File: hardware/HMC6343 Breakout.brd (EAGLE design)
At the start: 20.3 x 20.3 mm, 15 parts, among them U1 HMC6343A

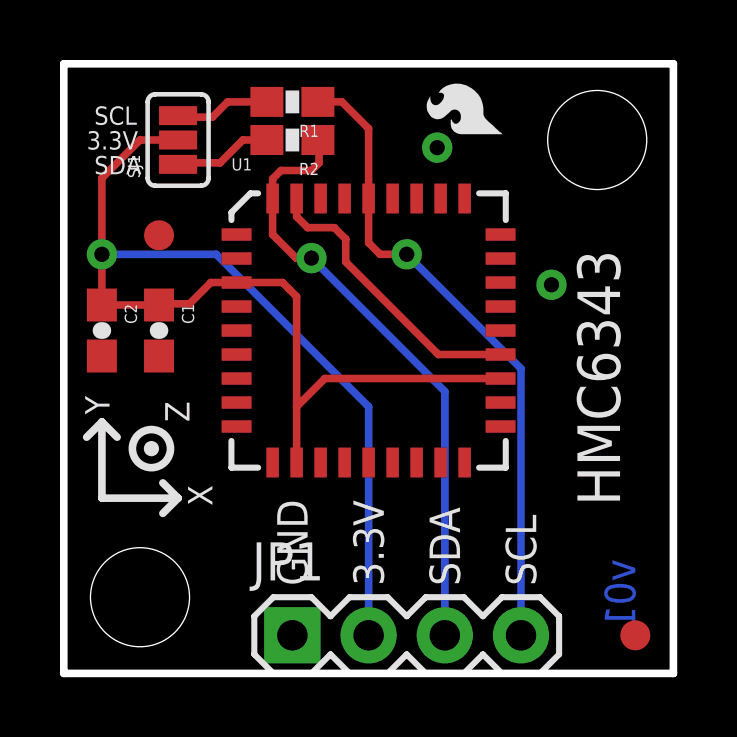
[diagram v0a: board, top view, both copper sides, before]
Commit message: v10, ready for reds
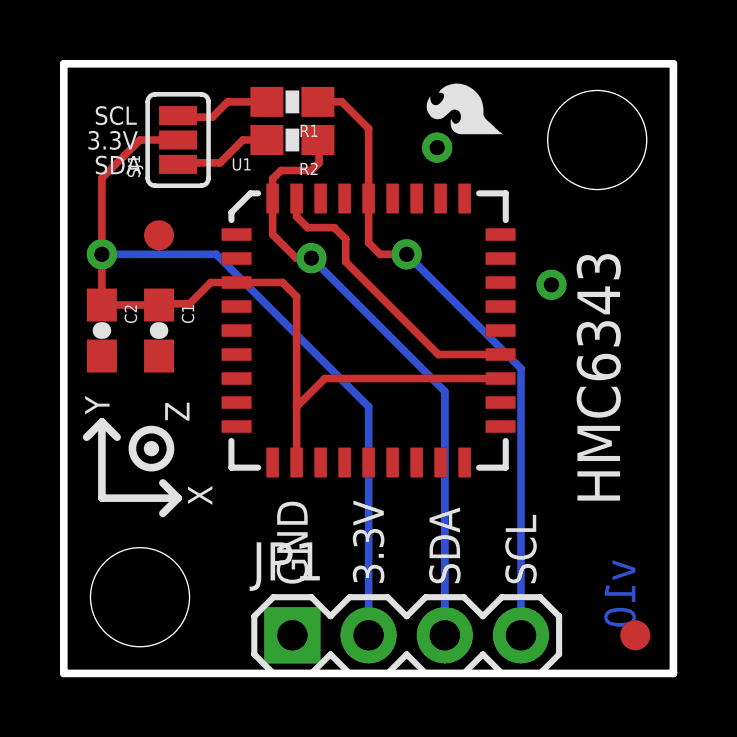
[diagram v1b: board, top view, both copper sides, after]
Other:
- board text added: "v10"
- board text removed: "v01"
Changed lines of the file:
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@@
 <text x="13.335" y="15.24" size="1.016" layer="22" font="vector" ratio="15" rot="SMR270">Magnetometer</text>
 <text x="14.986" y="13.462" size="1.016" layer="22" font="vector" ratio="15" rot="SMR270">Breakout</text>
-<text x="19.05" y="3.81" size="1.016" layer="16" font="vector" ratio="15" rot="SMR270">v01</text>
+<text x="19.05" y="3.81" size="1.016" layer="16" font="vector" ratio="15" rot="SMR270">v10</text>
 <wire x1="1.397" y1="16.256" x2="1.397" y2="18.796" width="0.254" layer="22"/>
 <wire x1="1.397" y1="16.256" x2="3.937" y2="16.256" width="0.254" layer="22"/>
